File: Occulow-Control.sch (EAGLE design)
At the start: 7 parts

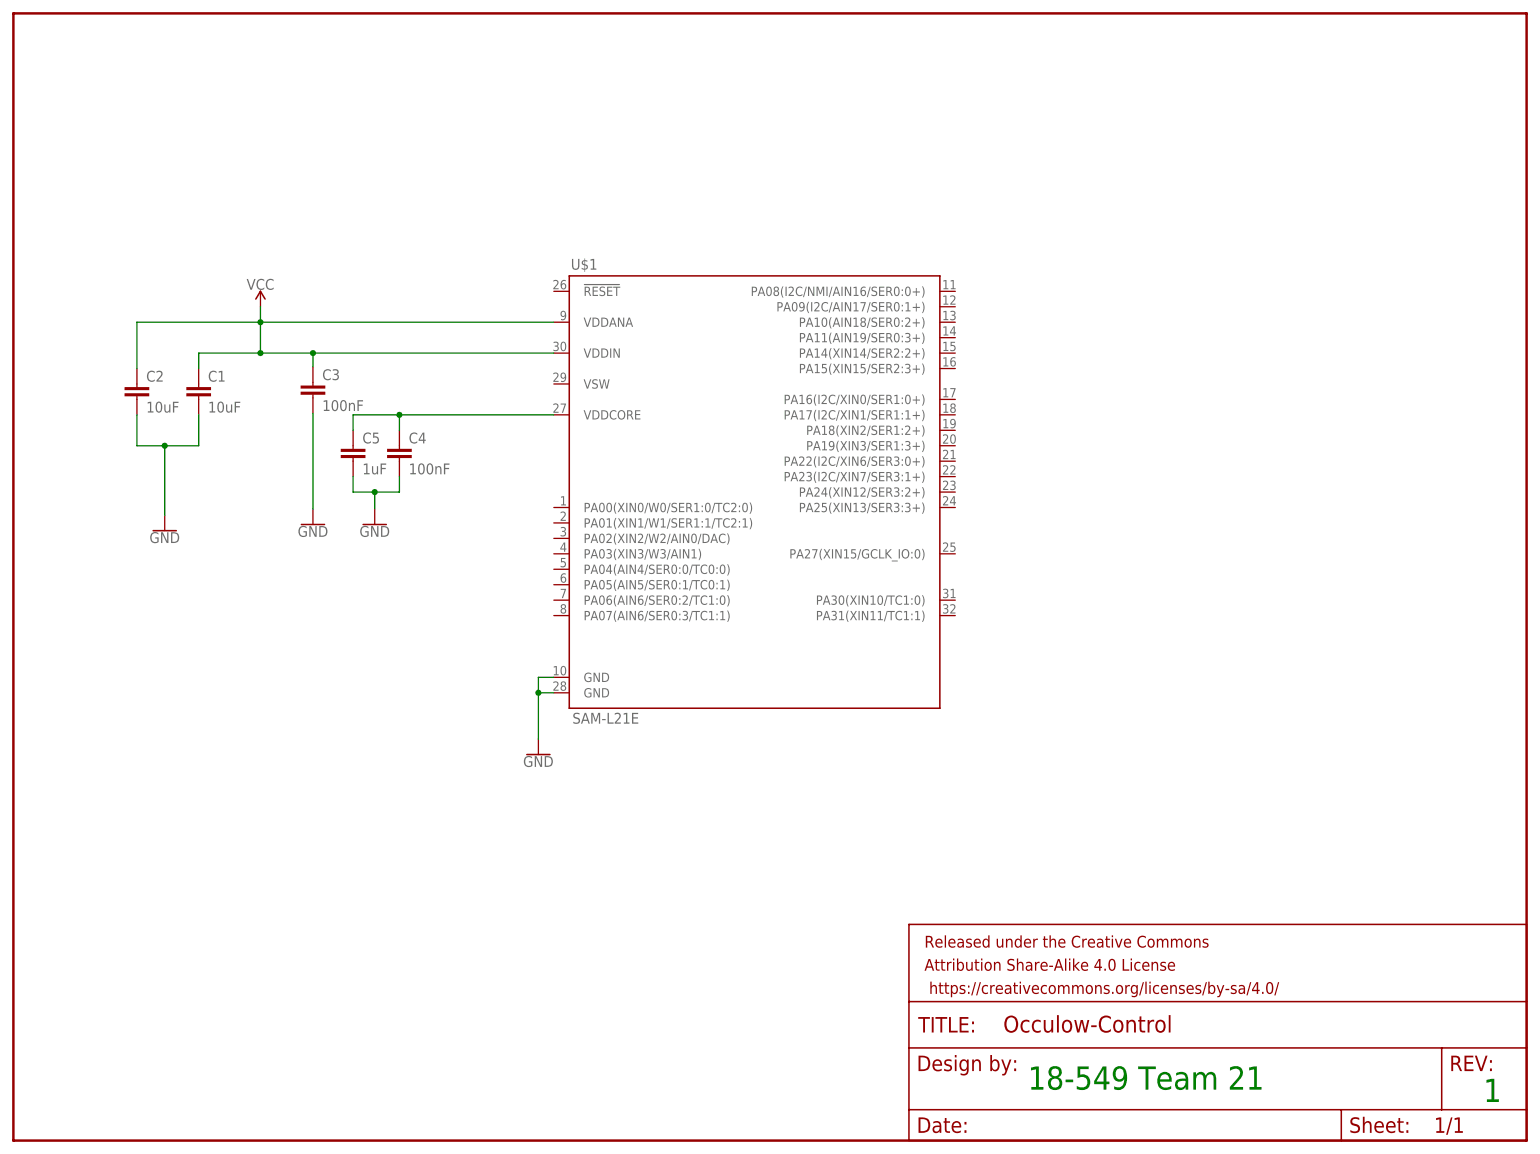
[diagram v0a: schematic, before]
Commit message: Port lora module
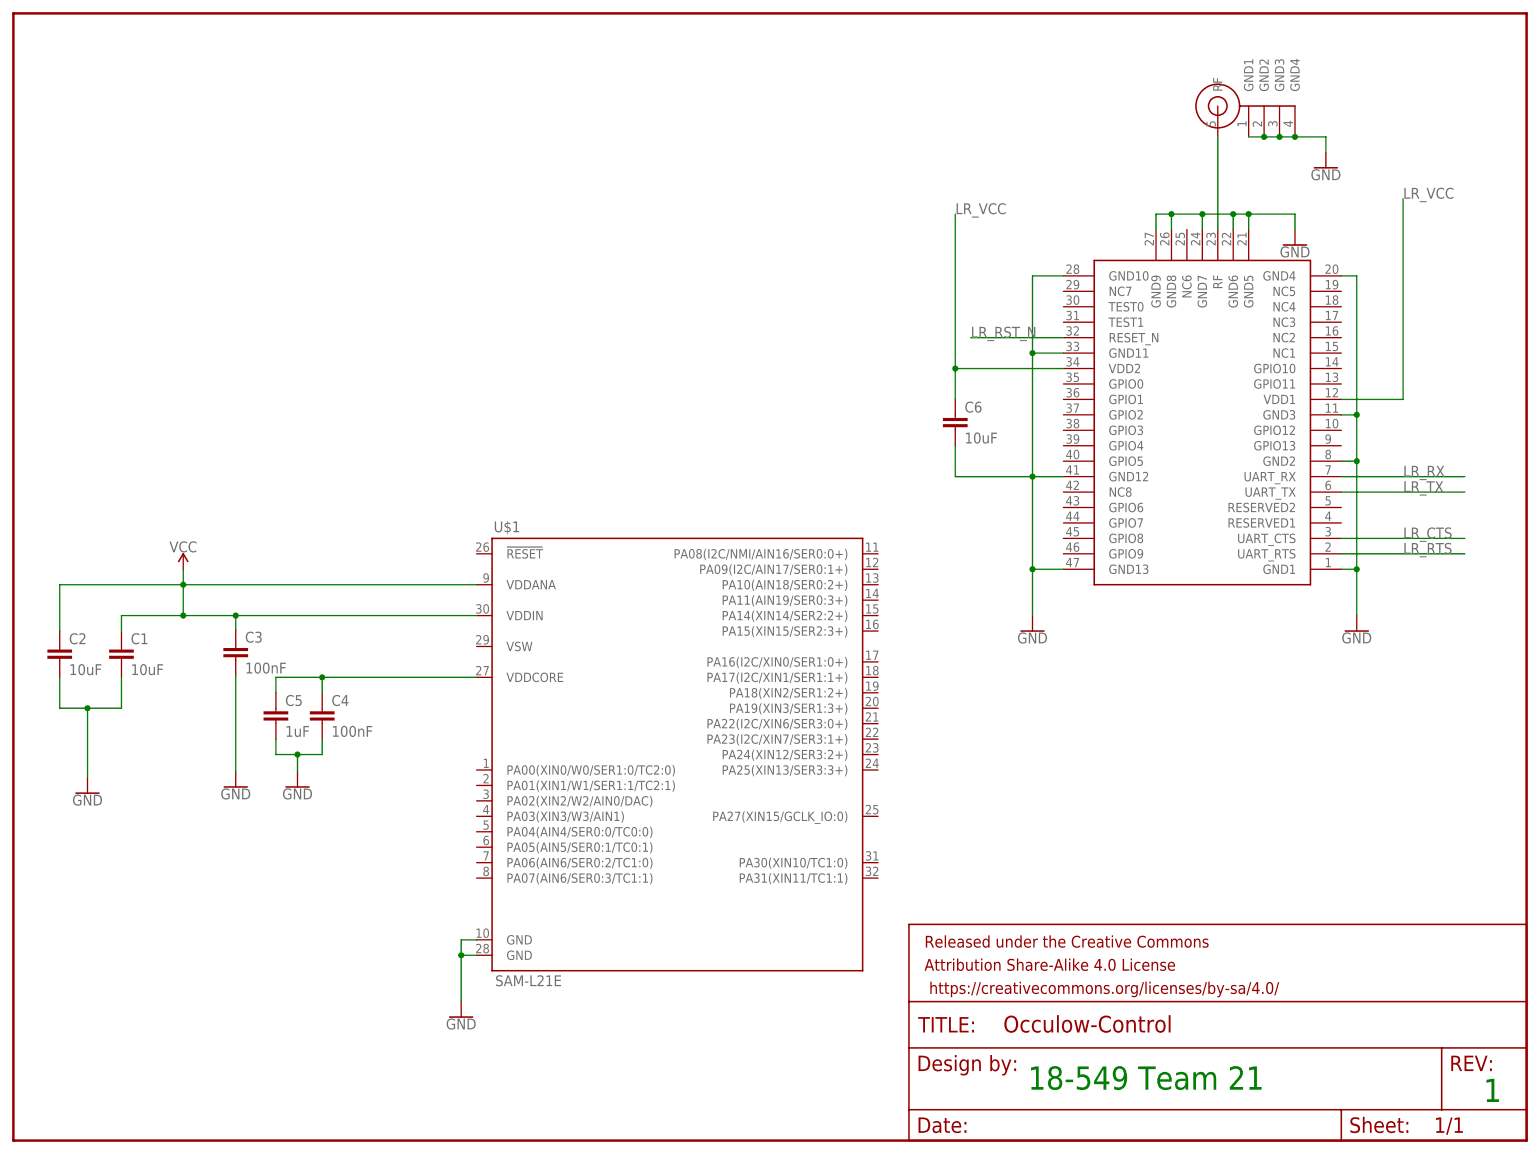
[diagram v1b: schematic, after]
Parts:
- added C6: 10uF, rcl:C-EUC1206
- added U$2: RN2903, RN2903:RN2903
- added U$3: SMA-JACKFEMALE, SMA-JACK:SMA-JACKFEMALE
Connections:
- new net LR_CTS: U$2.UART_CTS
- new net LR_RST_N: U$2.RESET_N
- new net LR_RTS: U$2.UART_RTS
- new net LR_RX: U$2.UART_RX
- new net LR_TX: U$2.UART_TX
- new net LR_VCC: C6.1, U$2.VDD1, U$2.VDD2
- new net RF: U$2.RF, U$3.RF
- net GND: now also C6.2, U$2.GND1, U$2.GND10, U$2.GND11, U$2.GND12, U$2.GND13, U$2.GND2, U$2.GND3, U$2.GND4, U$2.GND5, U$2.GND6, U$2.GND7, U$2.GND8, U$2.GND9, U$3.GND1, U$3.GND2, U$3.GND3, U$3.GND4
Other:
- moved on the sheet: C1, C2, C3, C4, C5, U$1
